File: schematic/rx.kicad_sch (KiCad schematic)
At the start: 34 parts, among them Q12 2N3904, U11 ADE-1L

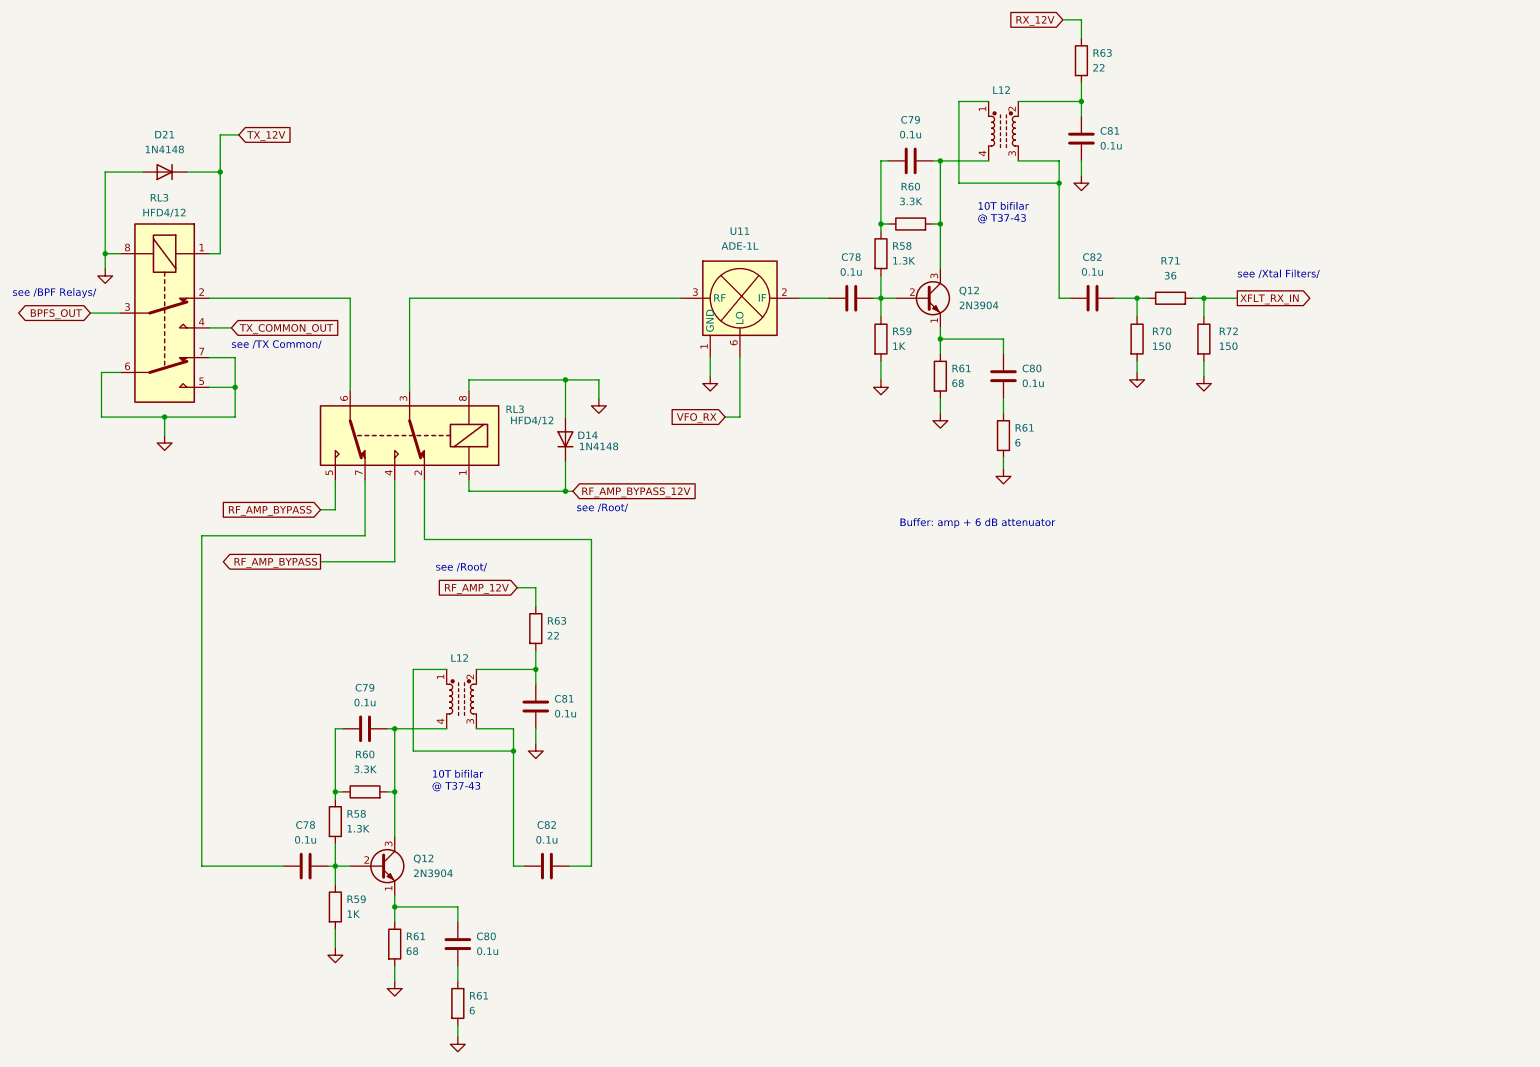
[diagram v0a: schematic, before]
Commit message: Minor changes
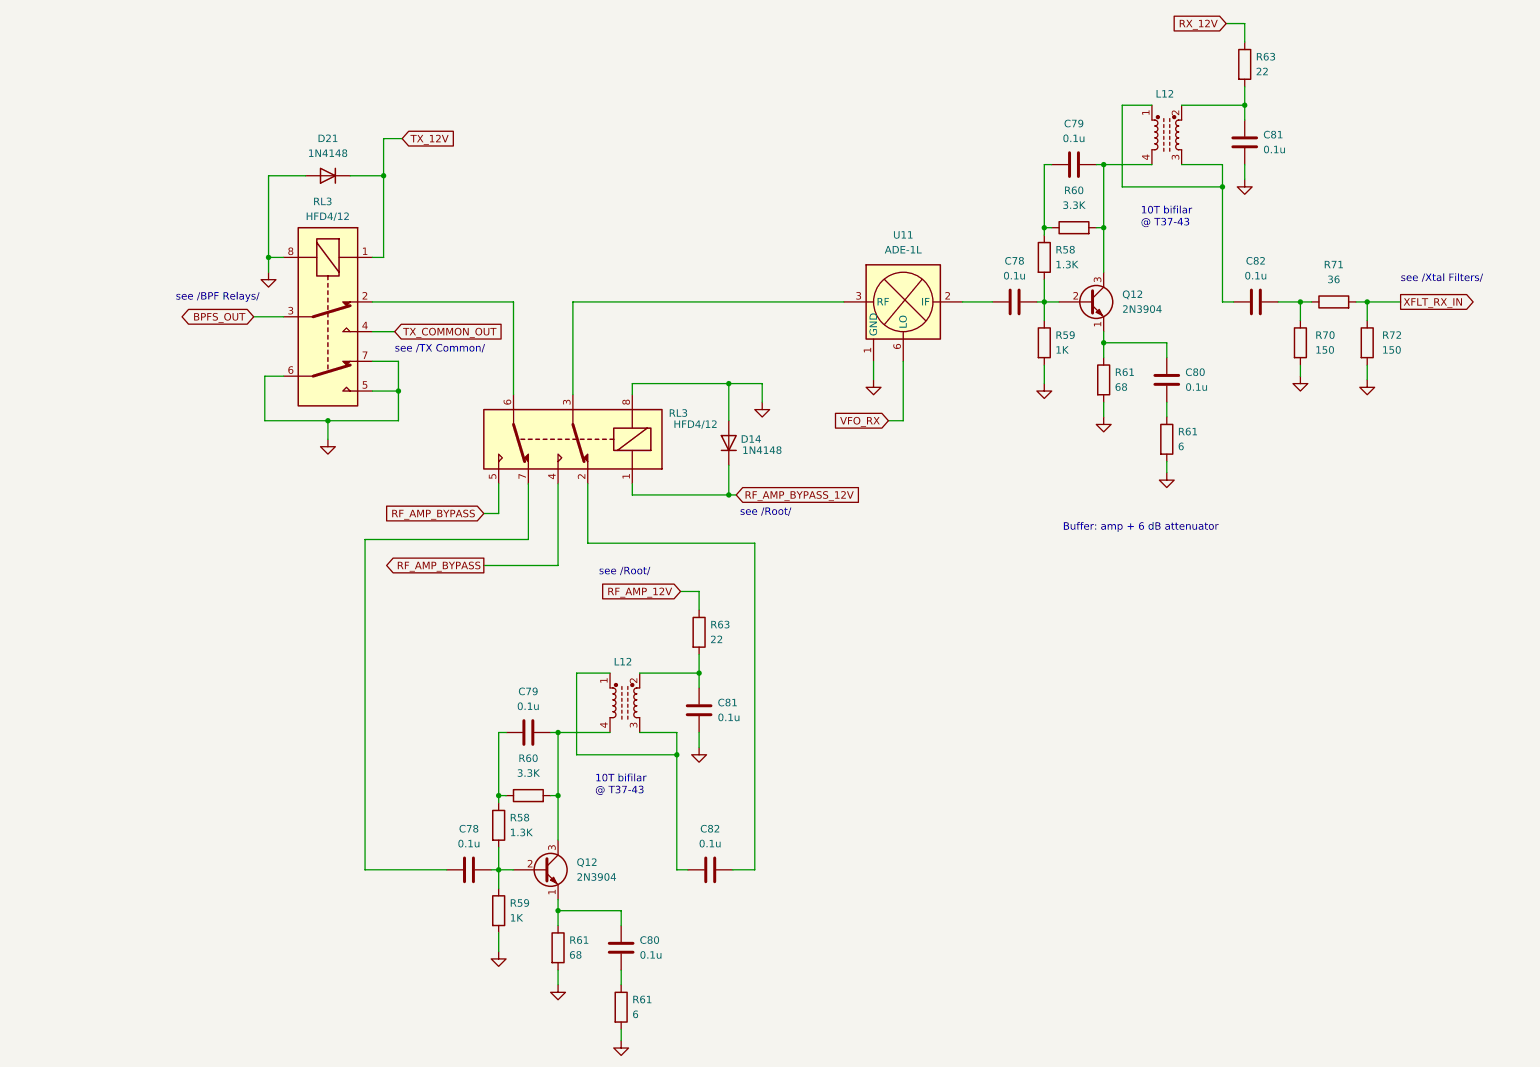
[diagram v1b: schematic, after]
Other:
- moved on the sheet: C78, C79, C80, C81, C82, D14, D21, L12, Q12, R58, R59, R60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
